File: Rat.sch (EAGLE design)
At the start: 37 parts, among them IC1 LM308N, Q1A 2N5458, Q1B MMBF5458

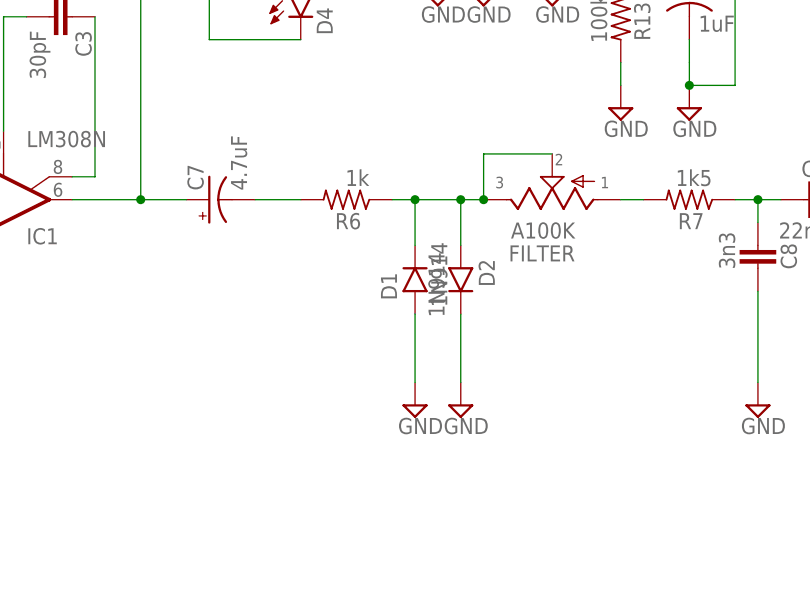
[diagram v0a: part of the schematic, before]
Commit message: Files for Seeed Studio
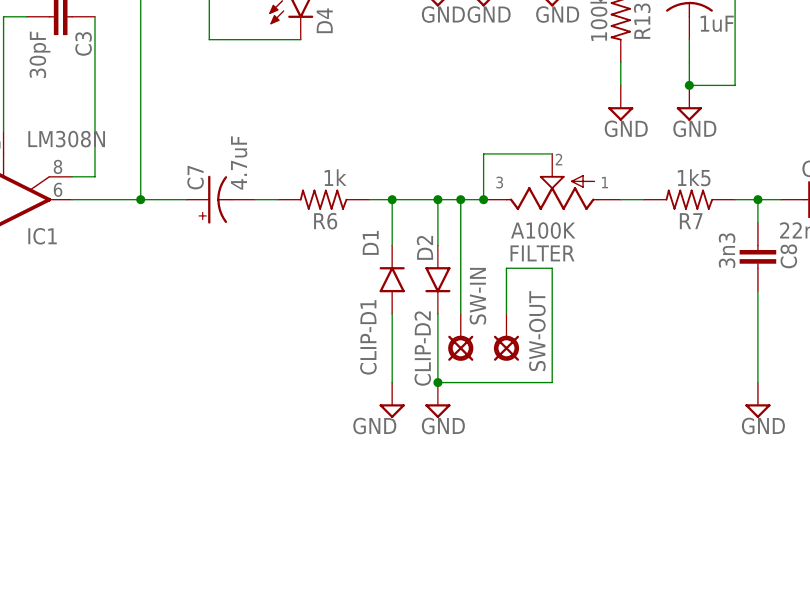
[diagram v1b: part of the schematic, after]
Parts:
- added SW-IN: (no value), mb_supply:PAD
- added SW-OUT: (no value), mb_supply:PADO
- D1: value 1N914 -> CLIP-D1
- D2: value 1N914 -> CLIP-D2
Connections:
- net GND: now also SW-OUT.PAD
- net N$11: now also SW-IN.PAD
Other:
- moved on the sheet: D1, D2, R6
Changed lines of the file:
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@@
 <part name="C2" library="mb_caps-box" deviceset="072X025" device="2" value="1nF"/>
 <part name="IC1" library="mb_ics" deviceset="LM308" device="N"/>
-<part name="D1" library="mb_diodes" deviceset="1N914" device=".3" value="1N914"/>
-<part name="D2" library="mb_diodes" deviceset="1N914" device=".3" value="1N914"/>
+<part name="D1" library="mb_diodes" deviceset="1N914" device=".3" value="CLIP-D1"/>
+<part name="D2" library="mb_diodes" deviceset="1N914" device=".3" value="CLIP-D2"/>
 <part name="D3" library="mb_diodes" deviceset="1N400X" device=".3" value="4002"/>
 <part name="C4" library="mb_caps-ceramic" deviceset="050X030_025" device="1" value="100pF"/>
@@
 <part name="GND10" library="mb_supply" deviceset="GND" device=""/>
 <part name="GND3" library="mb_supply" deviceset="GND" device=""/>
+<part name="SW-IN" library="mb_supply" deviceset="PAD" device=""/>
+<part name="SW-OUT" library="mb_supply" deviceset="PAD" device="O"/>
 </parts>
 <sheets>
@@
 <attribute name="VALUE" x="83.82" y="135.382" size="1.778" layer="96" rot="R180"/>
 </instance>
-<instance part="R6" gate="G$1" x="142.24" y="99.06" smashed="yes" rot="R180">
-<attribute name="NAME" x="143.891" y="97.5614" size="1.778" layer="95" rot="R180"/>
-<attribute name="VALUE" x="144.78" y="102.362" size="1.778" layer="96" rot="R180"/>
+<instance part="R6" gate="G$1" x="139.7" y="99.06" smashed="yes" rot="R180">
+<attribute name="NAME" x="141.351" y="97.5614" size="1.778" layer="95" rot="R180"/>
+<attribute name="VALUE" x="142.24" y="102.362" size="1.778" layer="96" rot="R180"/>
 </instance>
 <instance part="R7" gate="G$1" x="180.34" y="99.06" smashed="yes" rot="R180">
@@
 <attribute name="VALUE" x="231.775" y="73.025" size="1.778" layer="96"/>
 </instance>
-<instance part="GND8" gate="GND" x="154.94" y="76.2" smashed="yes">
-<attribute name="VALUE" x="153.035" y="73.025" size="1.778" layer="96"/>
+<instance part="GND8" gate="GND" x="152.4" y="76.2" smashed="yes">
+<attribute name="VALUE" x="150.495" y="73.025" size="1.778" layer="96"/>
 </instance>
 <instance part="GND9" gate="GND" x="91.44" y="76.2" smashed="yes">
@@
 <attribute name="VALUE" x="106.68" y="106.68" size="1.778" layer="96" rot="MR180"/>
 </instance>
-<instance part="D1" gate="G$1" x="149.86" y="91.44" smashed="yes" rot="R90">
-<attribute name="NAME" x="147.8534" y="87.884" size="1.778" layer="95" font="vector" rot="R90"/>
-<attribute name="VALUE" x="153.4414" y="87.122" size="1.778" layer="96" font="vector" rot="R90"/>
-</instance>
-<instance part="D2" gate="G$1" x="154.94" y="88.9" smashed="yes" rot="R270">
-<attribute name="NAME" x="156.9466" y="92.456" size="1.778" layer="95" font="vector" rot="R270"/>
-<attribute name="VALUE" x="151.3586" y="93.218" size="1.778" layer="96" font="vector" rot="R270"/>
+<instance part="D1" gate="G$1" x="147.32" y="91.44" smashed="yes" rot="R90">
+<attribute name="NAME" x="145.8214" y="92.71" size="1.778" layer="95" font="vector" rot="R90"/>
+<attribute name="VALUE" x="145.5674" y="79.502" size="1.778" layer="96" font="vector" rot="R90"/>
+</instance>
+<instance part="D2" gate="G$1" x="152.4" y="88.9" smashed="yes" rot="R270">
+<attribute name="NAME" x="150.0886" y="95.25" size="1.778" layer="95" font="vector" rot="R270"/>
+<attribute name="VALUE" x="149.8346" y="86.868" size="1.778" layer="96" font="vector" rot="R270"/>
 </instance>
 <instance part="D3" gate="1" x="152.4" y="134.62" smashed="yes" rot="R90">
@@
 <attribute name="VALUE" x="51.435" y="73.025" size="1.778" layer="96"/>
 </instance>
-<instance part="GND2" gate="GND" x="149.86" y="76.2" smashed="yes">
-<attribute name="VALUE" x="147.955" y="73.025" size="1.778" layer="96"/>
+<instance part="GND2" gate="GND" x="147.32" y="76.2" smashed="yes">
+<attribute name="VALUE" x="142.875" y="73.025" size="1.778" layer="96"/>
 </instance>
 <instance part="GND4" gate="GND" x="198.12" y="76.2" smashed="yes">
@@
 <instance part="GND3" gate="GND" x="101.6" y="116.84" smashed="yes" rot="R180">
 <attribute name="VALUE" x="103.505" y="120.015" size="1.778" layer="96" rot="R180"/>
+</instance>
+<instance part="SW-IN" gate="G$1" x="154.94" y="83.82" smashed="yes" rot="R270">
+<attribute name="NAME" x="155.956" y="91.694" size="1.778" layer="95" rot="R270"/>
+</instance>
+<instance part="SW-OUT" gate="G$1" x="160.02" y="83.82" smashed="yes" rot="R270">
+<attribute name="NAME" x="162.56" y="88.9" size="1.778" layer="95" rot="R270"/>
 </instance>
 </instances>
@@
 <pinref part="D2" gate="G$1" pin="C"/>
 <pinref part="GND8" gate="GND" pin="GND"/>
-<wire x1="154.94" y1="86.36" x2="154.94" y2="78.74" width="0.1524" layer="91"/>
+<wire x1="152.4" y1="86.36" x2="152.4" y2="78.74" width="0.1524" layer="91"/>
+<pinref part="SW-OUT" gate="G$1" pin="PAD"/>
+<wire x1="160.02" y1="86.36" x2="160.02" y2="91.44" width="0.1524" layer="91"/>
+<wire x1="160.02" y1="91.44" x2="165.1" y2="91.44" width="0.1524" layer="91"/>
+<wire x1="165.1" y1="91.44" x2="165.1" y2="78.74" width="0.1524" layer="91"/>
+<wire x1="165.1" y1="78.74" x2="152.4" y2="78.74" width="0.1524" layer="91"/>
+<junction x="152.4" y="78.74"/>
 </segment>
 <segment>
@@
 <segment>
 <pinref part="D1" gate="G$1" pin="A"/>
-<wire x1="149.86" y1="86.36" x2="149.86" y2="78.74" width="0.1524" layer="91"/>
+<wire x1="147.32" y1="86.36" x2="147.32" y2="78.74" width="0.1524" layer="91"/>
 <pinref part="GND2" gate="GND" pin="GND"/>
 </segment>
@@
 <pinref part="R6" gate="G$1" pin="2"/>
 <pinref part="C7" gate="1" pin="-"/>
-<wire x1="137.16" y1="99.06" x2="132.08" y2="99.06" width="0.1524" layer="91"/>
+<wire x1="134.62" y1="99.06" x2="132.08" y2="99.06" width="0.1524" layer="91"/>
 </segment>
 </net>
@@
 <pinref part="D1" gate="G$1" pin="C"/>
 <pinref part="R6" gate="G$1" pin="1"/>
-<wire x1="149.86" y1="93.98" x2="149.86" y2="99.06" width="0.1524" layer="91"/>
-<wire x1="149.86" y1="99.06" x2="147.32" y2="99.06" width="0.1524" layer="91"/>
+<wire x1="147.32" y1="93.98" x2="147.32" y2="99.06" width="0.1524" layer="91"/>
+<wire x1="147.32" y1="99.06" x2="144.78" y2="99.06" width="0.1524" layer="91"/>
 <pinref part="D2" gate="G$1" pin="A"/>
-<wire x1="154.94" y1="93.98" x2="154.94" y2="99.06" width="0.1524" layer="91"/>
-<wire x1="154.94" y1="99.06" x2="149.86" y2="99.06" width="0.1524" layer="91"/>
-<junction x="149.86" y="99.06"/>
+<wire x1="152.4" y1="93.98" x2="152.4" y2="99.06" width="0.1524" layer="91"/>
+<wire x1="152.4" y1="99.06" x2="147.32" y2="99.06" width="0.1524" layer="91"/>
+<junction x="147.32" y="99.06"/>
 <pinref part="FILTER" gate="G$1" pin="3"/>
 <wire x1="157.48" y1="99.06" x2="154.94" y2="99.06" width="0.1524" layer="91"/>
-<junction x="154.94" y="99.06"/>
+<junction x="152.4" y="99.06"/>
 <pinref part="FILTER" gate="G$1" pin="2"/>
+<wire x1="154.94" y1="99.06" x2="152.4" y2="99.06" width="0.1524" layer="91"/>
 <wire x1="157.48" y1="99.06" x2="157.48" y2="104.14" width="0.1524" layer="91"/>
 <wire x1="157.48" y1="104.14" x2="165.1" y2="104.14" width="0.1524" layer="91"/>
 <junction x="157.48" y="99.06"/>
-</segment>
-</net>
+<pinref part="SW-IN" gate="G$1" pin="PAD"/>
+<wire x1="154.94" y1="86.36" x2="154.94" y2="99.06" width="0.1524" layer="91"/>
+<junction x="154.94" y="99.06"/>
+</segment>
+</net>
